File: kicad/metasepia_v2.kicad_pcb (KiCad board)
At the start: 2 copper layers, 207.8 x 133.8 mm, 65 parts

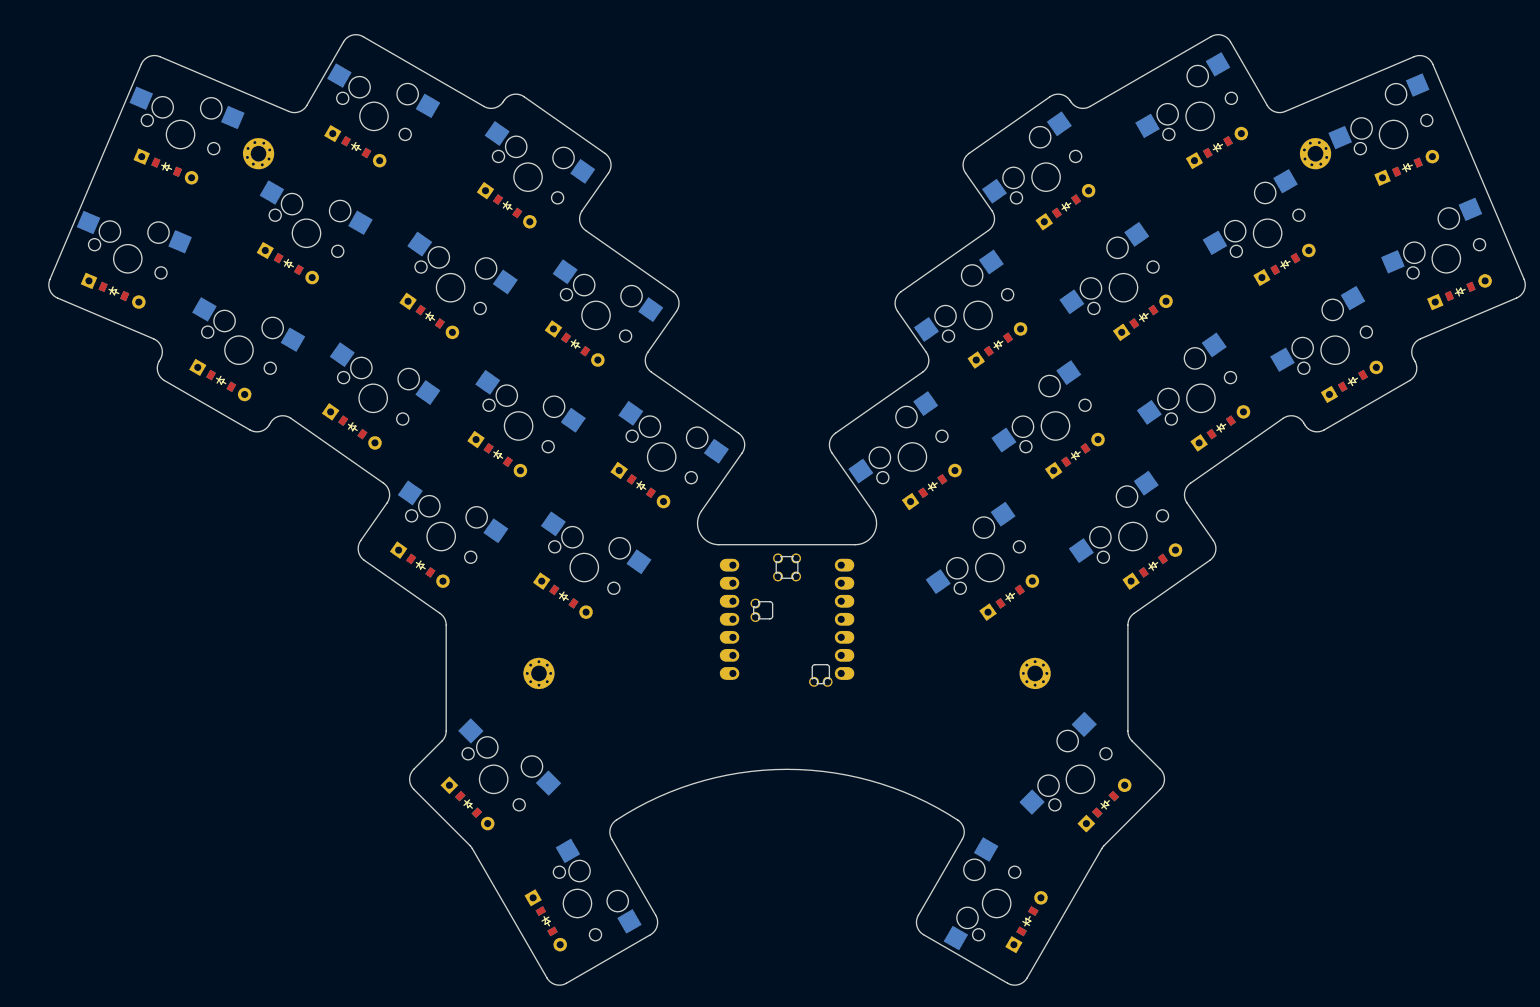
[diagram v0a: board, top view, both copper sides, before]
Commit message: fully route metasepiav2
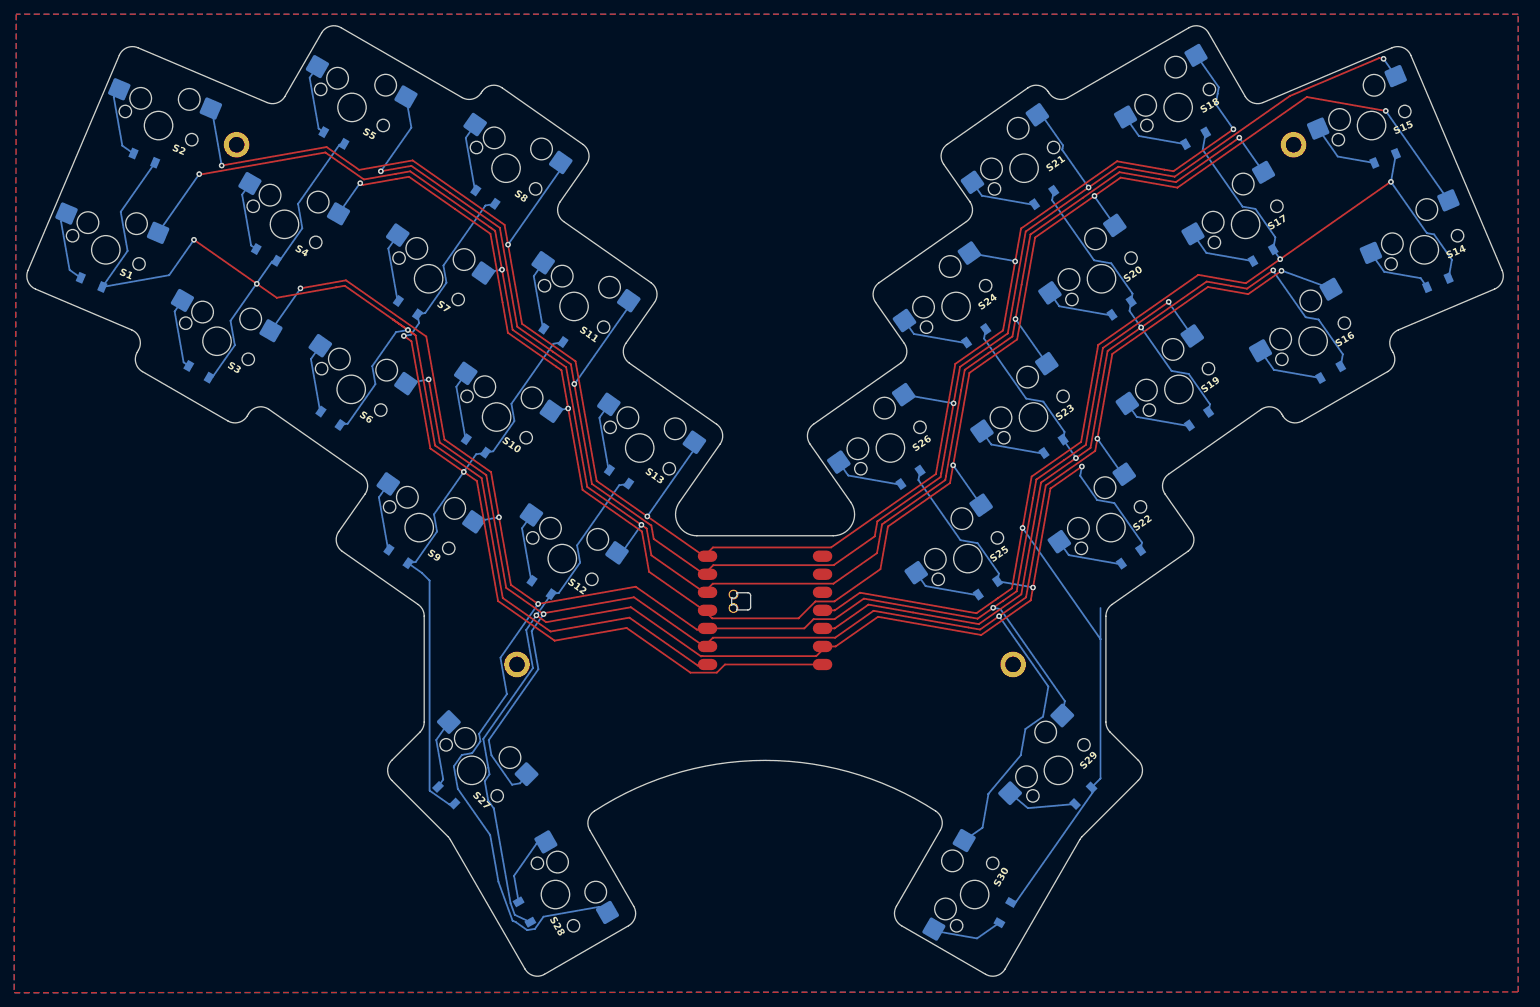
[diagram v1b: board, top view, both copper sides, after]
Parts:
- D1, D10, D11, D12, D13, D14, D15, D16, D17, D18, D19, D2, D20, D21, D22, D23, D24, D25, D26, D27, D28, D29, D3, D30, D4, D5, D6, D7, D8, D9: footprint ComboDiode -> frequent:diode
- S1, S10, S11, S12, S13, S14, S15, S16, S17, S18, S19, S2, S20, S21, S22, S23, S24, S25, S26, S27, S28, S29, S3, S30, S4, S5, S6, S7, S8, S9: footprint MX -> frequent:hsmx
- _1, _2, _3, _4: footprint m2hole -> frequent:m2hole
- moved S30 3.34 mm to (179.4, 148.0)
- moved S23 3.34 mm to (187.7, 80.8)
- moved D22 3.34 mm to (201.4, 100.5)
- moved MCU1 3.34 mm to (149.9, 108.0)
- moved D4 3.34 mm to (79.7, 58.0)
- moved S6 3.34 mm to (91.6, 76.9)
- moved S8 3.34 mm to (113.4, 45.8)
- moved S19 3.34 mm to (208.1, 76.9)
- moved S13 3.34 mm to (132.2, 85.2)
- moved D12 3.34 mm to (118.5, 104.8)
- moved D14 3.34 mm to (244.6, 61.9)
- moved S2 3.34 mm to (64.5, 39.8)
- moved D23 3.34 mm to (190.5, 84.9)
- moved D25 3.34 mm to (181.3, 104.8)
- moved D30 3.34 mm to (183.7, 150.5)
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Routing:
- net P4: track 0.00 -> 288.0 mm, vias 0 -> 5
- net P0: track 0.00 -> 266.3 mm, vias 0 -> 5
- net P5: track 0.00 -> 265.6 mm, vias 0 -> 5
- net P1: track 0.00 -> 265.3 mm, vias 0 -> 5
- net P3: track 0.00 -> 261.2 mm, vias 0 -> 5
- net P2: track 0.00 -> 255.2 mm, vias 0 -> 5
- net P10: track 0.00 -> 224.0 mm, vias 0 -> 3
- net P8: track 0.00 -> 211.2 mm, vias 0 -> 3
- net P6: track 0.00 -> 207.2 mm, vias 0 -> 3
- net P7: track 0.00 -> 195.5 mm, vias 0 -> 2
- net P9: track 0.00 -> 177.8 mm, vias 0 -> 3
- net reachy_default: track 0.00 -> 10.6 mm
- net pinky_top: track 0.00 -> 10.2 mm
- net pinky_home: track 0.00 -> 10.2 mm
- net mirror_reachy_default: track 0.00 -> 10.2 mm
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- added copper zone on B.Cu, net P0
- added copper zone on F.Cu, net P0
